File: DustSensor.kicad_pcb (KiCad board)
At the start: 2 copper layers, 20 parts, among them J1 UART_CONNECTOR, J2 USB_C_CONN, J3 SPS30_CONN, J4 OLED_CONN, SW1 RESET, SW2 BOOT, U1 ESP32-S3-WROOM-1, U2 AMS1117-3.3

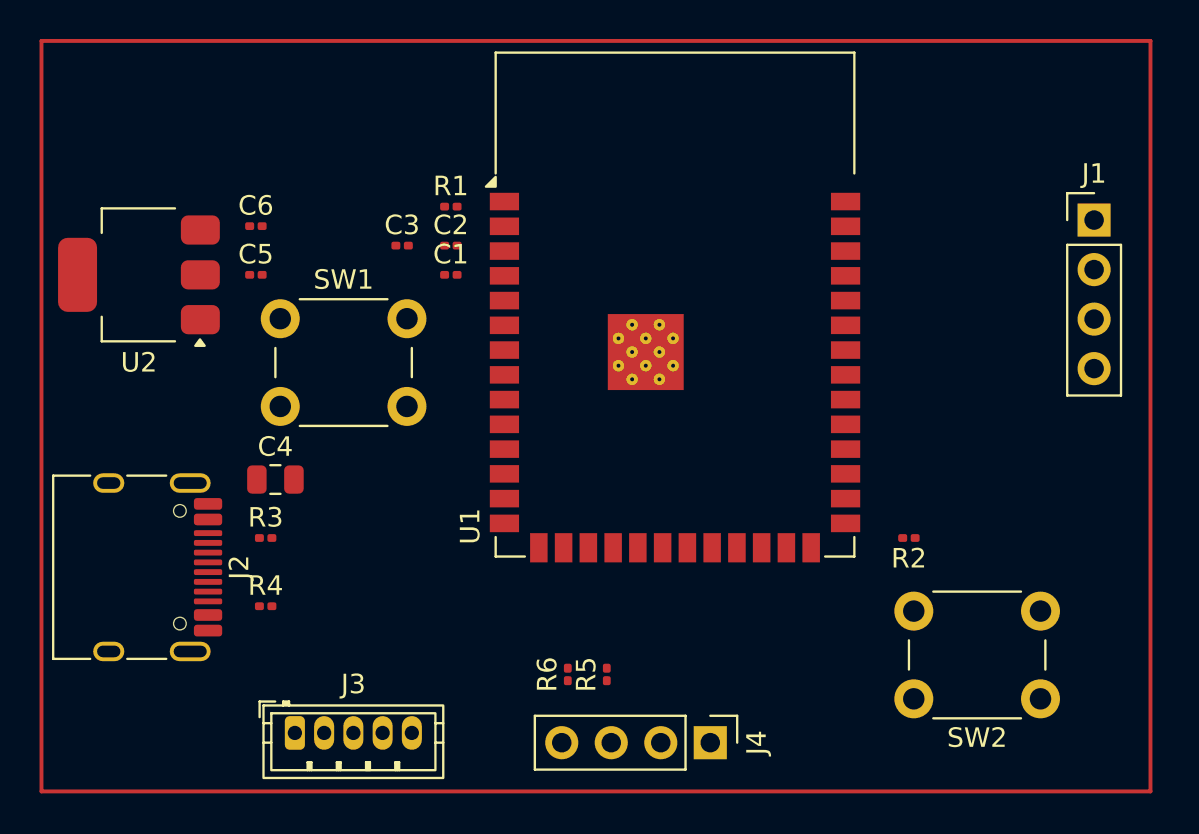
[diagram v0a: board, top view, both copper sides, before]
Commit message: Started routing
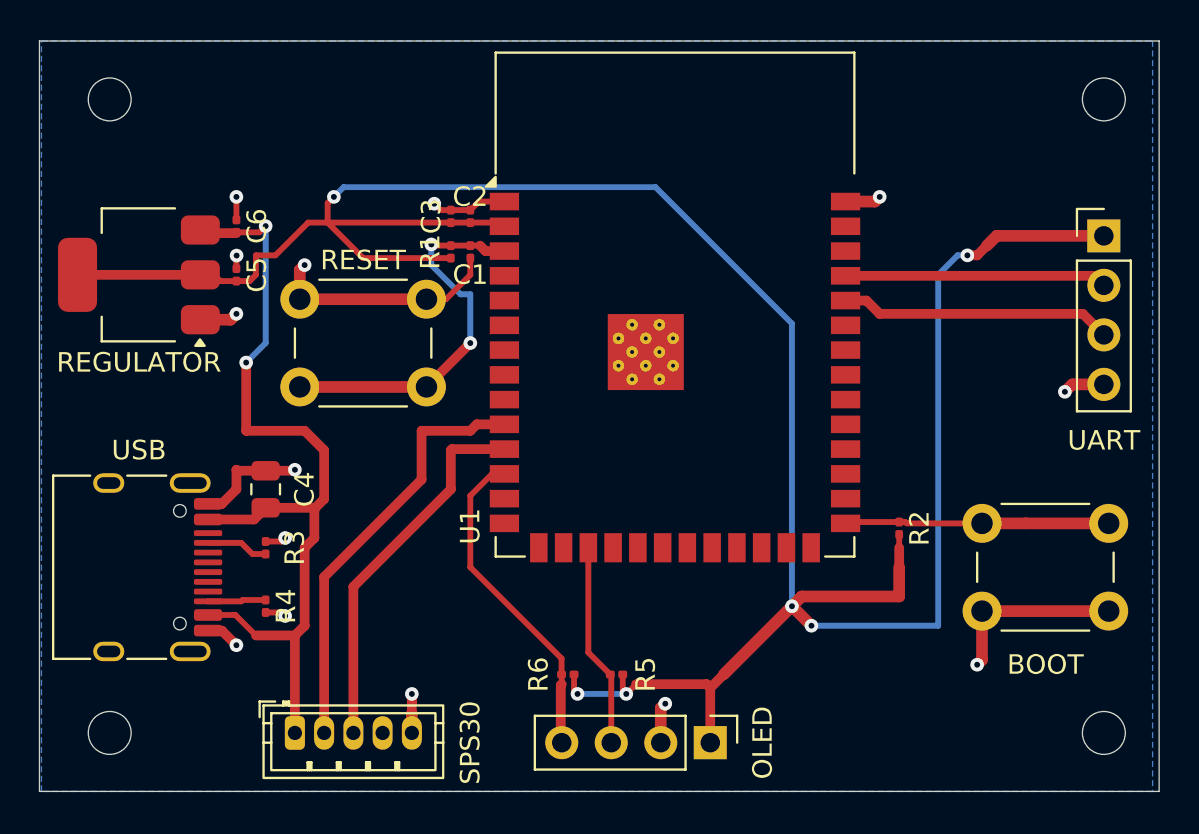
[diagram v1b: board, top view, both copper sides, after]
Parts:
- added REF: MountingHole_2.2mm_M2, MountingHole:MountingHole_2.2mm_M2, F.Cu at (125.0, 83.0)
- added REF**: MountingHole_2.2mm_M2, MountingHole:MountingHole_2.2mm_M2, F.Cu at (125.0, 115.5)
- added REF**: MountingHole_2.2mm_M2, MountingHole:MountingHole_2.2mm_M2, F.Cu at (176.0, 83.0)
- added REF**: MountingHole_2.2mm_M2, MountingHole:MountingHole_2.2mm_M2, F.Cu at (176.0, 115.5)
- moved BOOT 5.70 mm to (176.2, 109.2)
- moved C3 2.92 mm to (142.5, 89.0), turned to -90 degrees
- moved R1 2.32 mm to (142.5, 90.8), turned to 90 degrees
- moved C2 1.80 mm to (143.5, 89.0), turned to 90 degrees
- moved C1 1.55 mm to (143.5, 90.8), turned to 90 degrees
- moved RESET 1.41 mm to (134.8, 93.2)
- moved C5 1.00 mm to (131.5, 92.0), turned to -90 degrees
- moved C6 1.00 mm to (131.5, 89.5), turned to -90 degrees
- moved UART 0.95 mm to (176.0, 90.0)
- moved C4 0.71 mm to (133.0, 103.0), turned to 90 degrees
- moved R2 0.71 mm to (165.5, 105.0), turned to -90 degrees
- moved R3 0.50 mm to (133.0, 106.0), turned to 90 degrees
- moved R5 0.50 mm to (151.0, 112.5), turned to 180 degrees
- turned R4 to -90 degrees
- turned R6 to 180 degrees
- renumbered SW2 to BOOT, J4 to OLED, U2 to REGULATOR, SW1 to RESET, J3 to SPS30, J1 to UART, J2 to USB
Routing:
- net /3v3: track 0.00 -> 135.7 mm, vias 0 -> 6
- net GND: track 0.00 -> 47.4 mm, vias 0 -> 14
- net /5V: track 0.00 -> 44.6 mm, vias 0 -> 2
- net /SPS30RX: track 0.00 -> 22.0 mm
- net /OLED_SDA: track 0.00 -> 19.9 mm
- net Net-(U1-EN): track 0.00 -> 19.8 mm, vias 0 -> 2
- net /SPS30TX: track 0.00 -> 19.3 mm
- net /UART_TX: track 0.00 -> 14.0 mm
- net Net-(U1-IO0): track 0.00 -> 13.6 mm
- net /UART_RX: track 0.00 -> 13.5 mm
- net /OLED_SCL: track 0.00 -> 10.6 mm
- net Net-(J2-CC1): track 0.00 -> 3.19 mm
- net Net-(J2-CC2): track 0.00 -> 3.03 mm
- added copper zone on B.Cu, net GND
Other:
- board outline added: 57.4 x 38.5 mm
